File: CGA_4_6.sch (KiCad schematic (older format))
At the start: 16 parts, among them U1 74S112, U15 74LS00, U2 74LS74, U23 74LS32, U25 74LS00, U26 74S04, U27 74LS51, U28 74LS10, U29 74S04, U30 74LS32, U46 74LS00, U47 74LS51, U48 74LS51, U49 74LS02, U62 74LS125, U65 74LS02

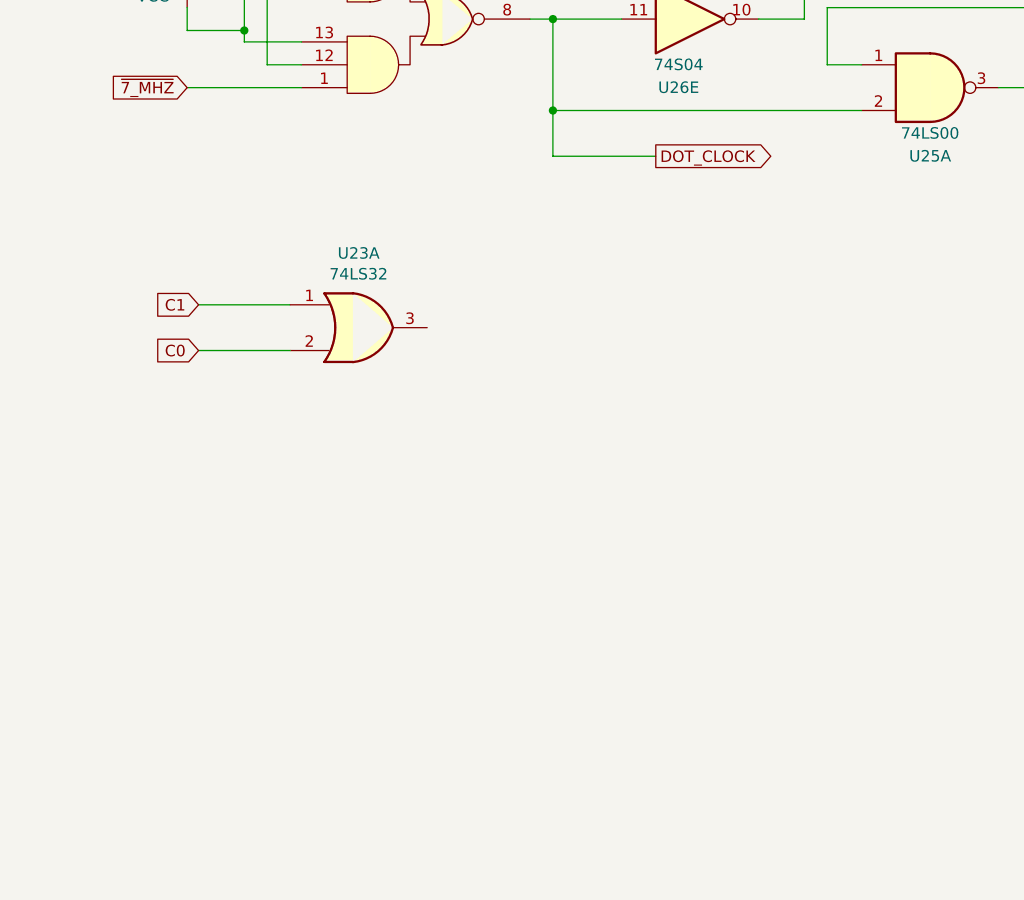
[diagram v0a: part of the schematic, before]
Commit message: More sheet 4
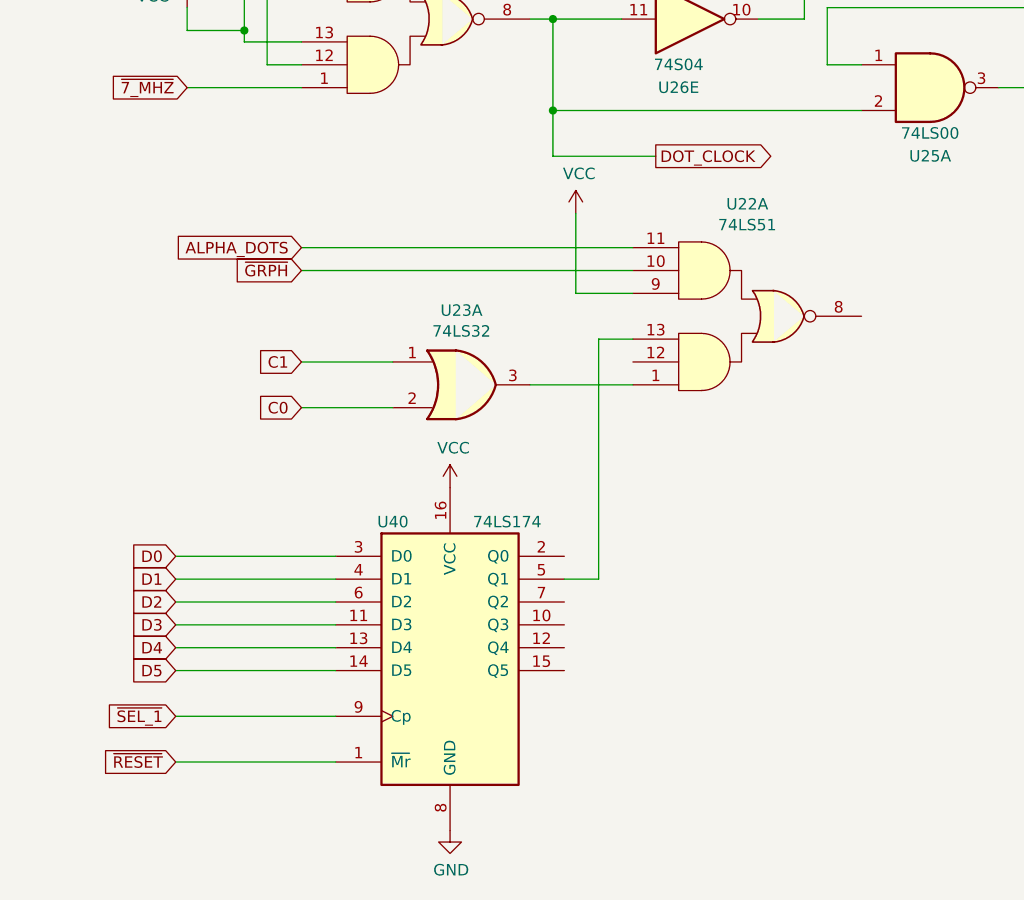
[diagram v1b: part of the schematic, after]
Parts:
- added U22: 74LS51, Package_DIP:DIP-14_W7.62mm_LongPads, symbol 74xx:74LS51
- added U40: 74LS174, Package_DIP:DIP-16_W7.62mm_LongPads, symbol 74xx:74LS174
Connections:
- net VCC: now also U22.9, U40.16 (VCC)
- net ~GRPH: now also U22.10
- net at U23.3: now also U22.1
- new net: U22.13, U40.5 (Q1)
- new net ALPHA_DOTS: U22.11
- new net D0: U40.3 (D0)
- new net D1: U40.4 (D1)
- new net D2: U40.6 (D2)
- new net D3: U40.11 (D3)
- new net D4: U40.13 (D4)
- new net D5: U40.14 (D5)
- new net GND: U40.8 (GND)
- new net ~RESET: U40.1 (~Mr)
- new net ~SEL_1: U40.9 (Cp)
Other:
- moved on the sheet: U23A
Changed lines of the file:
@@
 L 74xx:74LS32 U23
 U 1 1 6330493E
-P 1850 8600
-F 0 "U23" H 1850 8925 50  0000 C CNN
-F 1 "74LS32" H 1850 8834 50  0000 C CNN
-F 2 "Package_DIP:DIP-14_W7.62mm_LongPads" H 1850 8600 50  0001 C CNN
-F 3 "http://www.ti.com/lit/gpn/sn74LS32" H 1850 8600 50  0001 C CNN
-	1    1850 8600
+P 2300 8850
+F 0 "U23" H 2300 9175 50  0000 C CNN
+F 1 "74LS32" H 2300 9084 50  0000 C CNN
+F 2 "Package_DIP:DIP-14_W7.62mm_LongPads" H 2300 8850 50  0001 C CNN
+F 3 "http://www.ti.com/lit/gpn/sn74LS32" H 2300 8850 50  0001 C CNN
+	1    2300 8850
 	1    0    0    -1
 $EndComp
-Text GLabel 1150 8500 0    50   Input ~ 0
+Text GLabel 1600 8750 0    50   Input ~ 0
 C1
 Wire Wire Line
-	1150 8500 1550 8500
-Text GLabel 1150 8700 0    50   Input ~ 0
+	1600 8750 2000 8750
+Text GLabel 1600 8950 0    50   Input ~ 0
 C0
 Wire Wire Line
-	1150 8700 1550 8700
+	1600 8950 2000 8950
+$Comp
+L 74xx:74LS51 U22
+U 1 1 6337DF08
+P 3550 8550
+F 0 "U22" H 3550 8060 50  0000 C CNN
+F 1 "74LS51" H 3550 8151 50  0000 C CNN
+F 2 "Package_DIP:DIP-14_W7.62mm_LongPads" H 3550 8550 50  0001 C CNN
+F 3 "http://www.ti.com/lit/ds/symlink/sn74ls51.pdf" H 3550 8550 50  0001 C CNN
+	1    3550 8550
+	1    0    0    1
+$EndComp
+Wire Wire Line
+	2600 8850 3050 8850
+$Comp
+L power:VCC #PWR?
+U 1 1 633C357D
+P 2800 8100
+F 0 "#PWR?" H 2800 7950 50  0001 C CNN
+F 1 "VCC" H 2815 8273 50  0000 C CNN
+F 2 "" H 2800 8100 50  0001 C CNN
+F 3 "" H 2800 8100 50  0001 C CNN
+	1    2800 8100
+	1    0    0    -1
+$EndComp
+Wire Wire Line
+	3050 8450 2800 8450
+Wire Wire Line
+	2800 8450 2800 8100
+Wire Wire Line
+	3050 8350 1600 8350
+Text GLabel 1600 8350 0    50   Input ~ 0
+~GRPH
+Wire Wire Line
+	3050 8250 1600 8250
+Text GLabel 1600 8250 0    50   Input ~ 0
+ALPHA_DOTS
+$Comp
+L 74xx:74LS174 U40
+U 1 1 63419162
+P 2250 10000
+F 0 "U40" H 2000 10550 50  0000 C CNN
+F 1 "74LS174" H 2500 10550 50  0000 C CNN
+F 2 "Package_DIP:DIP-16_W7.62mm_LongPads" H 2250 10000 50  0001 C CNN
+F 3 "http://www.ti.com/lit/gpn/sn74LS174" H 2250 10000 50  0001 C CNN
+	1    2250 10000
+	1    0    0    -1
+$EndComp
+$Comp
+L power:VCC #PWR?
+U 1 1 6341CA1D
+P 2250 9300
+F 0 "#PWR?" H 2250 9150 50  0001 C CNN
+F 1 "VCC" H 2265 9473 50  0000 C CNN
+F 2 "" H 2250 9300 50  0001 C CNN
+F 3 "" H 2250 9300 50  0001 C CNN
+	1    2250 9300
+	1    0    0    -1
+$EndComp
+$Comp
+L power:GND #PWR?
+U 1 1 6341DF93
+P 2250 10800
+F 0 "#PWR?" H 2250 10550 50  0001 C CNN
+F 1 "GND" H 2255 10627 50  0000 C CNN
+F 2 "" H 2250 10800 50  0001 C CNN
+F 3 "" H 2250 10800 50  0001 C CNN
+	1    2250 10800
+	1    0    0    -1
+$EndComp
+Text GLabel 1050 10300 0    50   Input ~ 0
+~SEL_1
+Wire Wire Line
+	1050 10300 1750 10300
+Text GLabel 1050 10500 0    50   Input ~ 0
+~RESET
+Wire Wire Line
+	1050 10500 1750 10500
+Wire Wire Line
+	1750 9600 1050 9600
+Wire Wire Line
+	1750 9700 1050 9700
+Wire Wire Line
+	1750 9800 1050 9800
+Wire Wire Line
+	1750 9900 1050 9900
+Wire Wire Line
+	1750 10000 1050 10000
+Wire Wire Line
+	1750 10100 1050 10100
+Text GLabel 1050 9600 0    50   Input ~ 0
+D0
+Text GLabel 1050 9700 0    50   Input ~ 0
+D1
+Text GLabel 1050 9800 0    50   Input ~ 0
+D2
+Text GLabel 1050 9900 0    50   Input ~ 0
+D3
+Text GLabel 1050 10000 0    50   Input ~ 0
+D4
+Text GLabel 1050 10100 0    50   Input ~ 0
+D5
+Wire Wire Line
+	3050 8650 2900 8650
+Wire Wire Line
+	2900 8650 2900 9700
+Wire Wire Line
+	2900 9700 2750 9700
 $EndSCHEMATC
